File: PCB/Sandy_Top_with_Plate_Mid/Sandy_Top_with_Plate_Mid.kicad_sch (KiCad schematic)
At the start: 75 parts, among them J1 Conn_02x02_Top_Bottom, J2 Conn_02x02_Top_Bottom, J3 Conn_02x02_Top_Bottom

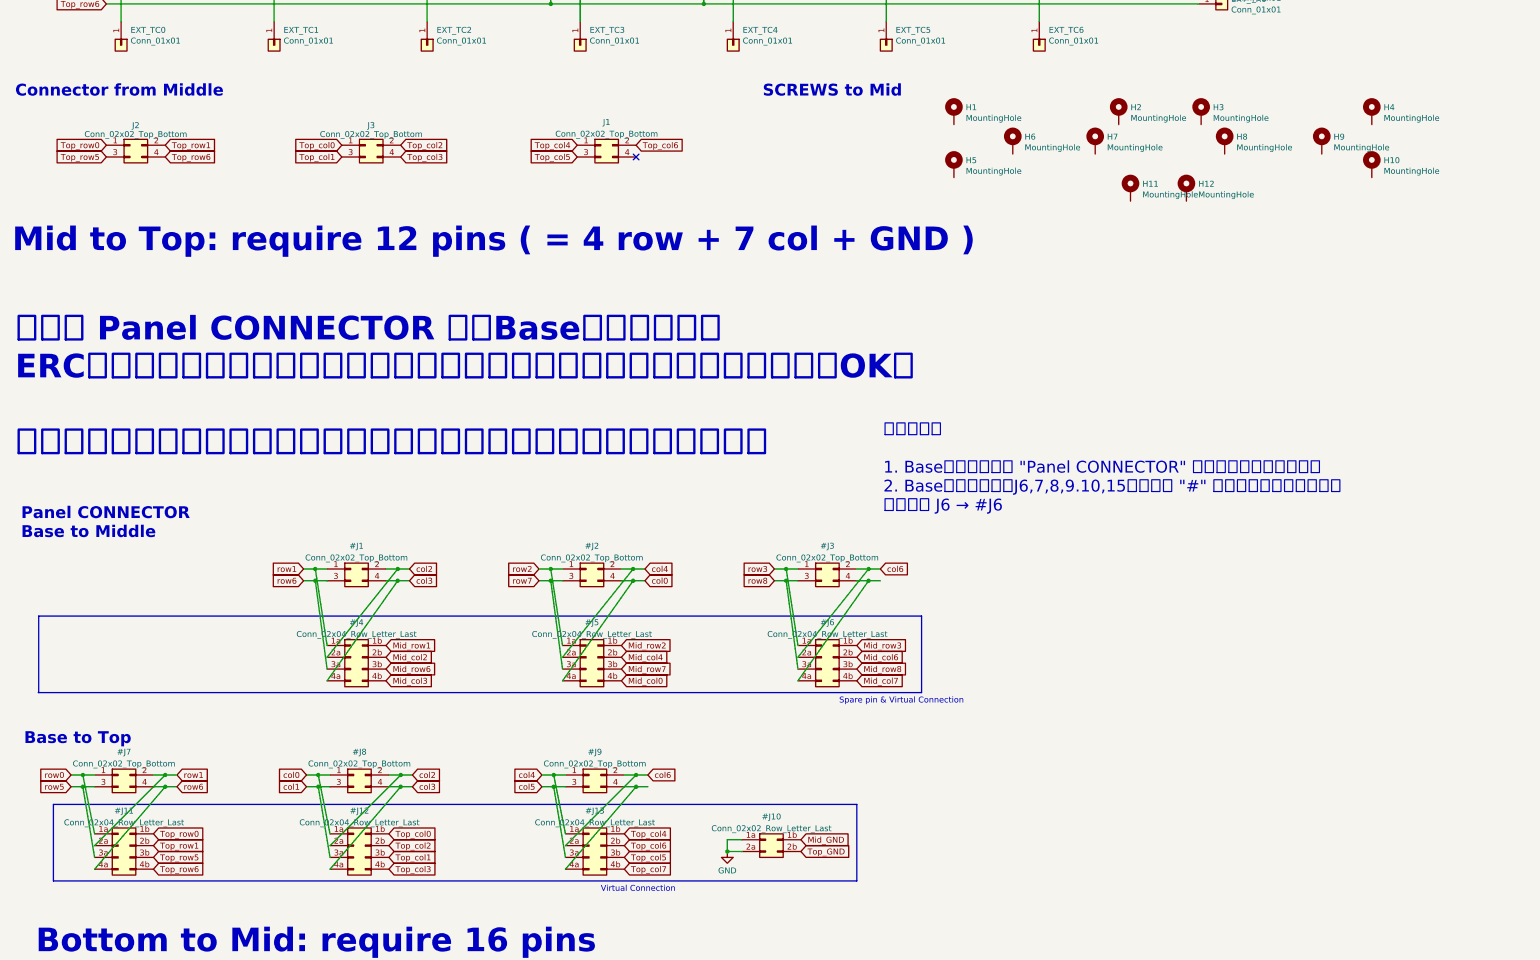
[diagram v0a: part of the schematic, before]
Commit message: 基板間ピン割り当て
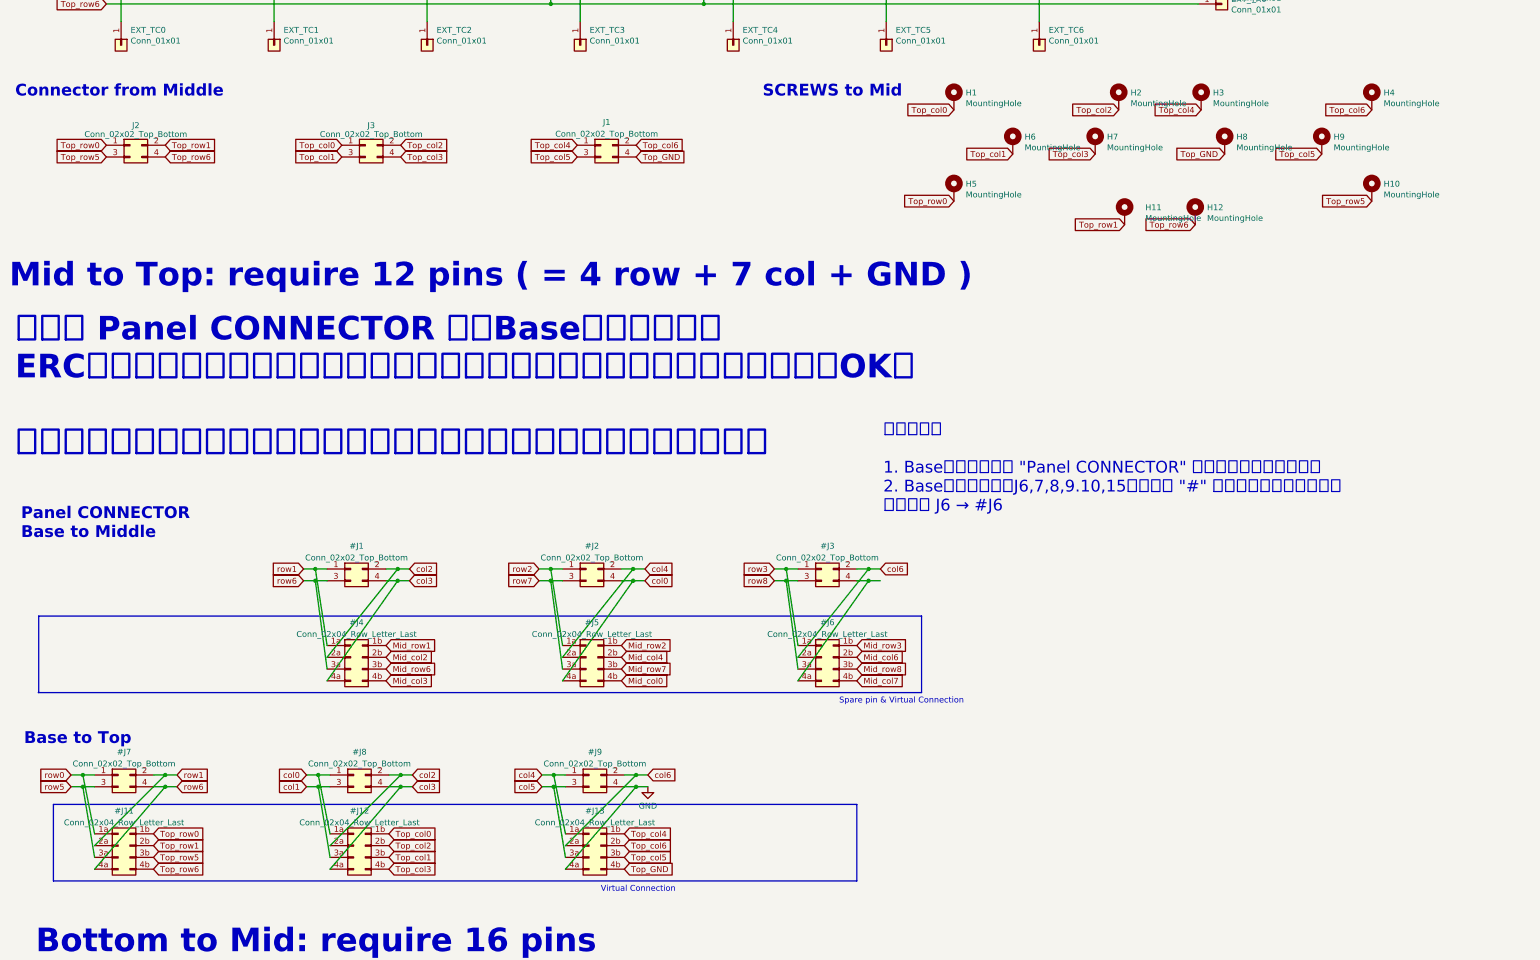
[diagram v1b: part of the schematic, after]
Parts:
- removed #J10: Conn_02x02_Row_Letter_Last, symbol Connector_Generic:Conn_02x02_Row_Letter_Last
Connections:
- net Top_col7 is gone; now on net Top_GND: #J13.4b (Pin_4b)
- net GND: now also #J13.4a (Pin_4a), #J9.4 (Pin_4)
- net Top_GND: now also H8.1, J1.4 (Pin_4)
- net Top_col0: now also H1.1
- net Top_col1: now also H6.1
- net Top_col2: now also H2.1
- net Top_col3: now also H7.1
- net Top_col4: now also H3.1
- net Top_col5: now also H9.1
- net Top_col6: now also H4.1
- net Top_row0: now also H5.1
- net Top_row1: now also H11.1
- net Top_row5: now also H10.1
- net Top_row6: now also H12.1
- no-connect marks 1 -> 0
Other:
- moved on the sheet: H1, H10, H11, H12, H2, H3, H4, H5
